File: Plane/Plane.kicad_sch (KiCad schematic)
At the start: 18 parts, among them M1 Aileron_Left, M2 Aileron_Right, M3 Elevator, M4 Rudder, M5 Speed Controller, M6 Unassigned, M7 Unassigned, M8 Unassigned

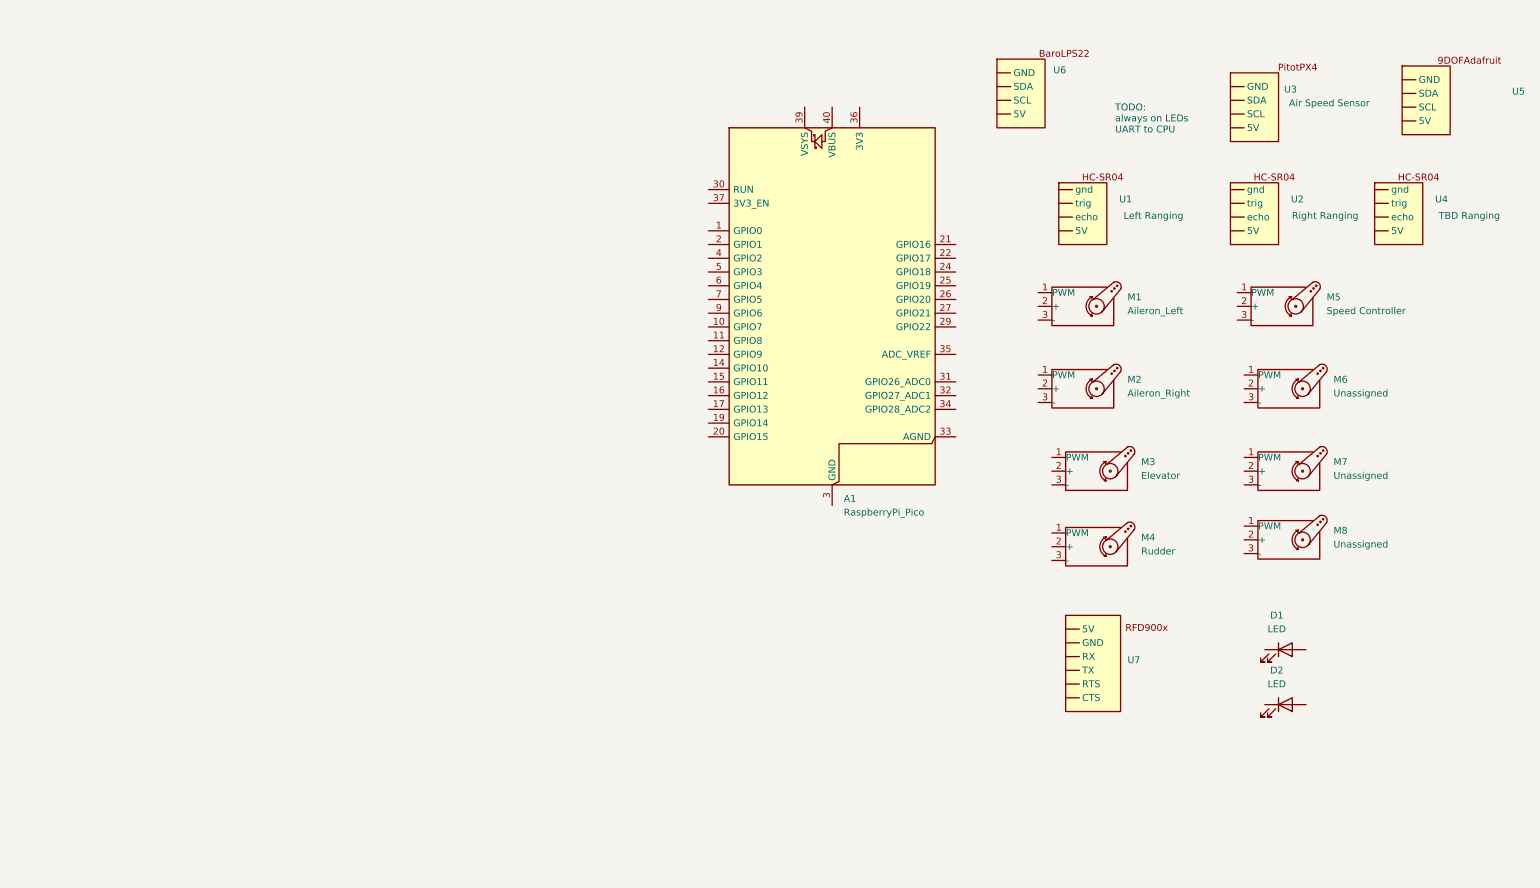
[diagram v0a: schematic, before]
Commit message: schematic
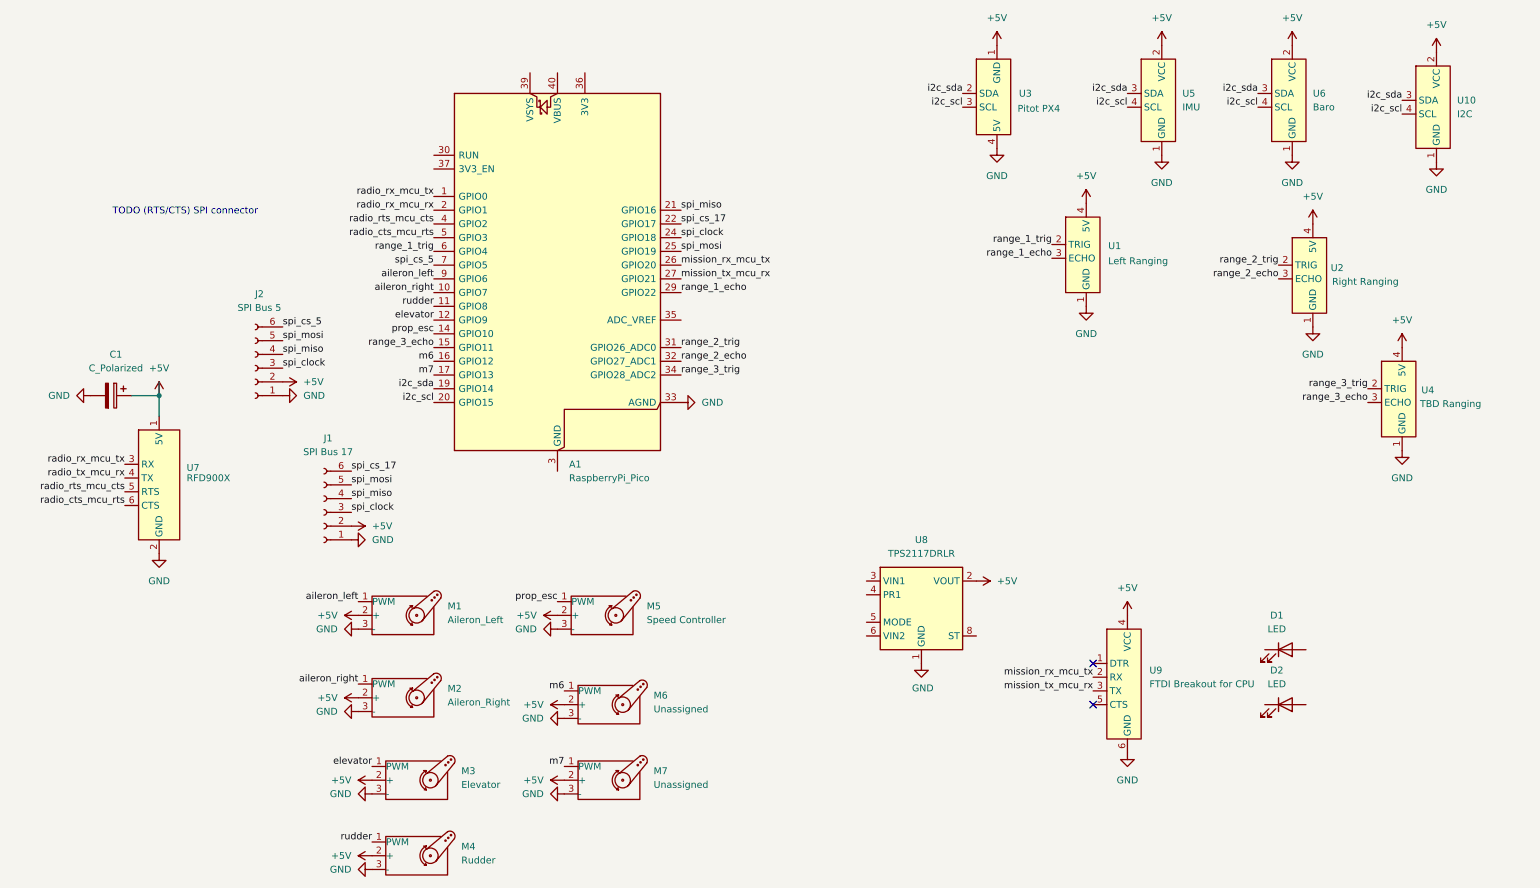
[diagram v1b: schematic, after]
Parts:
- removed M6: Unassigned, symbol Motor:Motor_Servo
- removed U5: ~, symbol Sensor_Motion:9DOFI2c
- removed U6: ~, symbol Sensor_Motion:BaroLPS22
- added C1: C_Polarized, symbol Device:C_Polarized
- added J1: SPI Bus 17, symbol Connector:Conn_01x06_Socket
- added J2: SPI Bus 5, symbol Connector:Conn_01x06_Socket
- added U10: I2C, symbol Connector:STEMMA
- added U5: IMU, symbol Connector:STEMMA
- added U6: Baro, symbol Connector:STEMMA
- added U8: TPS2117DRLR, Package_TO_SOT_SMD:SOT-583-8, symbol Power_Management:TPS2117DRLR
- added U9: FTDI Breakout for CPU, symbol Connector:YP-05-FTDI-Breakout
- U1: value ~ -> Left Ranging
- U2: value ~ -> Right Ranging
- U3: value ~ -> Pitot PX4
- U4: value ~ -> TBD Ranging
- U7: value ~ -> RFD900X
- renumbered M8 to M6
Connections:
- net m6: now reaches M6.1 (PWM)
- net m6: now also A1.16 (GPIO12)
- net +5V: now reaches M6.2 (+)
- net +5V: now also M1.2 (+), M2.2 (+), M3.2 (+), M4.2 (+), M5.2 (+), M7.2 (+), U1.4 (5V), U2.4 (5V), U3.1 (GND), U4.4 (5V), U7.1 (5V), C1.1, J1.2 (Pin_2), J2.2 (Pin_2), U10.2 (VCC), U5.2 (VCC), U6.2 (VCC), U8.2 (VOUT), U8.7 (VOUT), U9.4 (VCC)
- net GND: now reaches M6.3 (-)
- net GND: now also A1.33 (AGND), M1.3 (-), M2.3 (-), M3.3 (-), M4.3 (-), M5.3 (-), M7.3 (-), U1.1 (GND), U2.1 (GND), U3.4 (5V), U4.1 (GND), U7.2 (GND), C1.2, J1.1 (Pin_1), J2.1 (Pin_1), U10.1 (GND), U5.1 (GND), U6.1 (GND), U8.1 (GND), U9.6 (GND)
- net rudder: now reaches M4.1 (PWM)
- net rudder: now also A1.11 (GPIO8)
- net radio_rx_mcu_tx: now reaches A1.1 (GPIO0)
- net radio_rx_mcu_tx: now also U7.3 (RX)
- net aileron_right: now reaches A1.10 (GPIO7)
- net aileron_right: now also M2.1 (PWM)
- net elevator: now reaches A1.12 (GPIO9)
- net elevator: now also M3.1 (PWM)
- net prop_esc: now reaches A1.14 (GPIO10)
- net prop_esc: now also M5.1 (PWM)
- net range_3_echo: now reaches A1.15 (GPIO11)
- net range_3_echo: now also U4.3 (ECHO)
- net m7: now reaches A1.17 (GPIO13)
- net m7: now also M7.1 (PWM)
- net i2c_sda: now reaches A1.19 (GPIO14)
- net i2c_sda: now also U3.2 (SDA), U10.3 (SDA), U5.3 (SDA), U6.3 (SDA)
- net radio_rx_mcu_rx: now reaches A1.2 (GPIO1)
- net i2c_scl: now reaches A1.20 (GPIO15)
- net i2c_scl: now also U3.3 (SCL), U10.4 (SCL), U5.4 (SCL), U6.4 (SCL)
- net spi_miso: now reaches A1.21 (GPIO16)
- net spi_miso: now also J1.4 (Pin_4), J2.4 (Pin_4)
- net spi_cs_17: now reaches A1.22 (GPIO17)
- net spi_cs_17: now also J1.6 (Pin_6)
- net spi_clock: now reaches A1.24 (GPIO18)
- net spi_clock: now also J1.3 (Pin_3), J2.3 (Pin_3)
- net spi_mosi: now reaches A1.25 (GPIO19)
- net spi_mosi: now also J1.5 (Pin_5), J2.5 (Pin_5)
- net mission_rx_mcu_tx: now reaches A1.26 (GPIO20)
- net mission_rx_mcu_tx: now also U9.2 (RX)
- net mission_tx_mcu_rx: now reaches A1.27 (GPIO21)
- net mission_tx_mcu_rx: now also U9.3 (TX)
- net range_1_echo: now reaches A1.29 (GPIO22)
- net range_1_echo: now also U1.3 (ECHO)
- net range_2_trig: now reaches A1.31 (GPIO26_ADC0)
- net range_2_trig: now also U2.2 (TRIG)
- net range_2_echo: now reaches A1.32 (GPIO27_ADC1)
- net range_2_echo: now also U2.3 (ECHO)
- net range_3_trig: now reaches A1.34 (GPIO28_ADC2)
- net range_3_trig: now also U4.2 (TRIG)
- net radio_rts_mcu_cts: now reaches A1.4 (GPIO2)
- net radio_rts_mcu_cts: now also U7.5 (RTS)
- net radio_cts_mcu_rts: now reaches A1.5 (GPIO3)
- net radio_cts_mcu_rts: now also U7.6 (CTS)
- net range_1_trig: now reaches A1.6 (GPIO4)
- net range_1_trig: now also U1.2 (TRIG)
- net spi_cs_5: now reaches A1.7 (GPIO5)
- net spi_cs_5: now also J2.6 (Pin_6)
- net aileron_left: now reaches A1.9 (GPIO6)
- net aileron_left: now also M1.1 (PWM)
- new net radio_tx_mcu_rx: U7.4 (TX)
- no-connect marks 0 -> 2
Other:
- note added: "TODO (RTS/CTS) SPI connector"
- note removed: "TODO: always on LEDs UART to CPU"
- moved on the sheet: A1, M1, M2, M3, M4, M5, M6, M7
